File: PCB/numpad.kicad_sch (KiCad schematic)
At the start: 72 parts, among them J1 AVR-ISP-6, J2 Conn_01x04_Female, SW1 SW_Push, U1 ProMicro

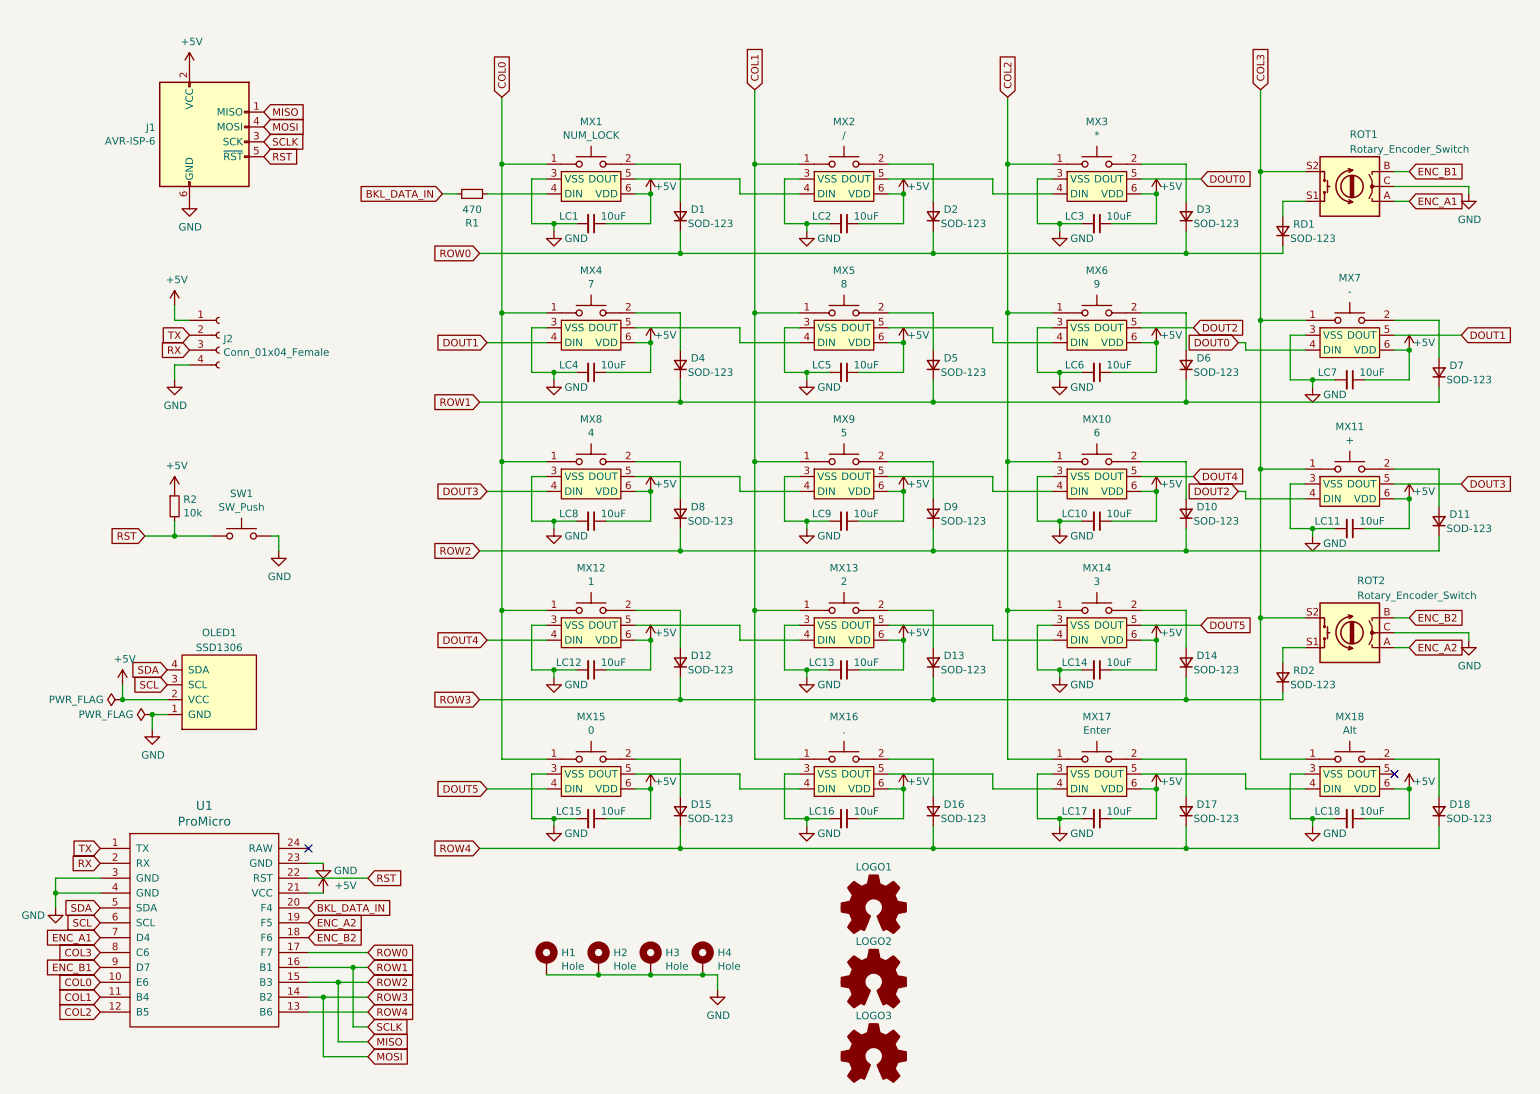
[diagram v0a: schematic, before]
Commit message: Completely redid schematic and PCB
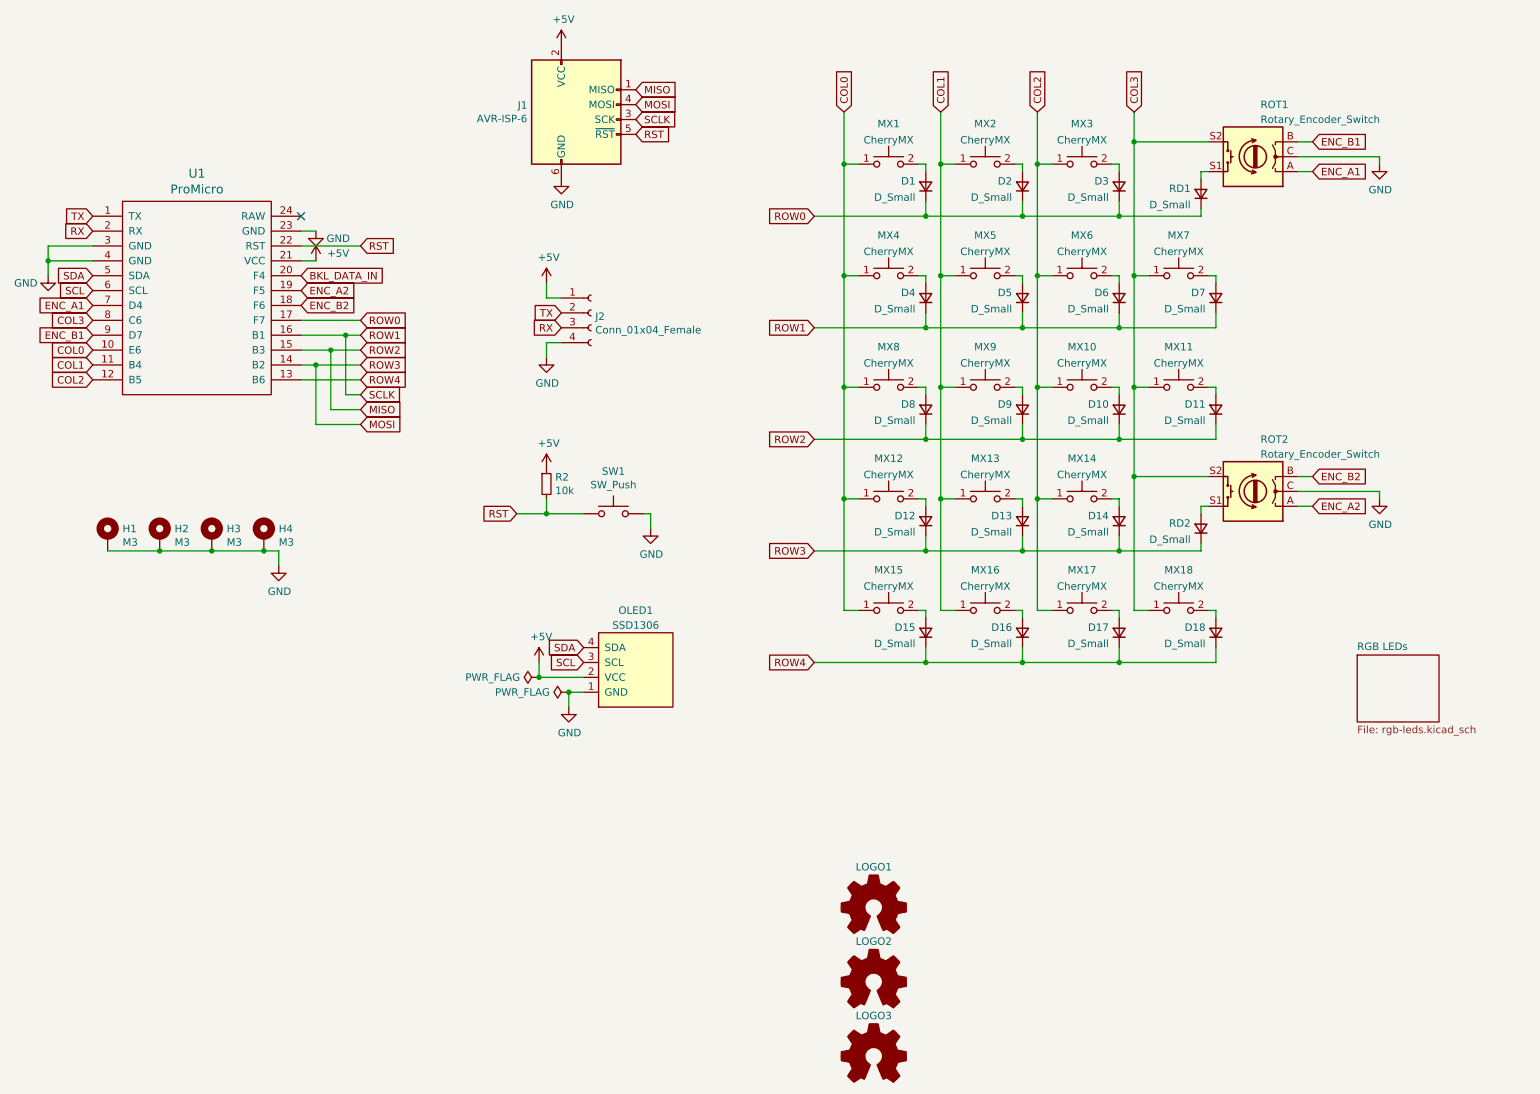
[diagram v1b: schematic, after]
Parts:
- removed LC1, LC10, LC11, LC12, LC13, LC14, LC15, LC16, LC17, LC18, LC2, LC3, LC4, LC5, LC6, LC7, LC8, LC9: 10uF, Capacitor_SMD:C_0805_2012Metric, symbol Device:C_Small
- removed MX1: NUM_LOCK, CherryMX_PCB_KailhSocket_LTST-A683CEGBW:CherryMX_1.00u_PCB_KailhSocket_LTST-A683CEGBW, symbol CherryMX:CherryMX_LTST-A683CEGBW
- removed MX10: 6, CherryMX_PCB_KailhSocket_LTST-A683CEGBW:CherryMX_1.00u_PCB_KailhSocket_LTST-A683CEGBW, symbol CherryMX:CherryMX_LTST-A683CEGBW
- removed MX11: +, CherryMX_PCB_KailhSocket_StabWireBottom_LTST-A683CEGBW:CherryMX_2.00u_PCB_KailhSocket_StabWireBottom_LTST-A683CEGBW, symbol CherryMX:CherryMX_LTST-A683CEGBW
- removed MX12: 1, CherryMX_PCB_KailhSocket_LTST-A683CEGBW:CherryMX_1.00u_PCB_KailhSocket_LTST-A683CEGBW, symbol CherryMX:CherryMX_LTST-A683CEGBW
- removed MX13: 2, CherryMX_PCB_KailhSocket_LTST-A683CEGBW:CherryMX_1.00u_PCB_KailhSocket_LTST-A683CEGBW, symbol CherryMX:CherryMX_LTST-A683CEGBW
- removed MX14: 3, CherryMX_PCB_KailhSocket_LTST-A683CEGBW:CherryMX_1.00u_PCB_KailhSocket_LTST-A683CEGBW, symbol CherryMX:CherryMX_LTST-A683CEGBW
- removed MX15: 0, CherryMX_PCB_KailhSocket_StabWireBottom_LTST-A683CEGBW:CherryMX_2.00u_PCB_KailhSocket_StabWireBottom_LTST-A683CEGBW, symbol CherryMX:CherryMX_LTST-A683CEGBW
- removed MX16: ., CherryMX_PCB_KailhSocket_LTST-A683CEGBW:CherryMX_1.00u_PCB_KailhSocket_LTST-A683CEGBW, symbol CherryMX:CherryMX_LTST-A683CEGBW
- removed MX17: Enter, CherryMX_PCB_KailhSocket_StabWireBottom_LTST-A683CEGBW:CherryMX_2.00u_PCB_KailhSocket_StabWireBottom_LTST-A683CEGBW, symbol CherryMX:CherryMX_LTST-A683CEGBW
- removed MX18: Alt, CherryMX_PCB_KailhSocket_LTST-A683CEGBW:CherryMX_1.50u_PCB_KailhSocket_LTST-A683CEGBW, symbol CherryMX:CherryMX_LTST-A683CEGBW
- removed MX2: /, CherryMX_PCB_KailhSocket_LTST-A683CEGBW:CherryMX_1.00u_PCB_KailhSocket_LTST-A683CEGBW, symbol CherryMX:CherryMX_LTST-A683CEGBW
- removed MX3: *, CherryMX_PCB_KailhSocket_LTST-A683CEGBW:CherryMX_1.00u_PCB_KailhSocket_LTST-A683CEGBW, symbol CherryMX:CherryMX_LTST-A683CEGBW
- removed MX4: 7, CherryMX_PCB_KailhSocket_LTST-A683CEGBW:CherryMX_1.00u_PCB_KailhSocket_LTST-A683CEGBW, symbol CherryMX:CherryMX_LTST-A683CEGBW
- removed MX5: 8, CherryMX_PCB_KailhSocket_LTST-A683CEGBW:CherryMX_1.00u_PCB_KailhSocket_LTST-A683CEGBW, symbol CherryMX:CherryMX_LTST-A683CEGBW
- removed MX6: 9, CherryMX_PCB_KailhSocket_LTST-A683CEGBW:CherryMX_1.00u_PCB_KailhSocket_LTST-A683CEGBW, symbol CherryMX:CherryMX_LTST-A683CEGBW
- removed MX7: -, CherryMX_PCB_KailhSocket_LTST-A683CEGBW:CherryMX_1.00u_PCB_KailhSocket_LTST-A683CEGBW, symbol CherryMX:CherryMX_LTST-A683CEGBW
- removed MX8: 4, CherryMX_PCB_KailhSocket_LTST-A683CEGBW:CherryMX_1.00u_PCB_KailhSocket_LTST-A683CEGBW, symbol CherryMX:CherryMX_LTST-A683CEGBW
- removed MX9: 5, CherryMX_PCB_KailhSocket_LTST-A683CEGBW:CherryMX_1.00u_PCB_KailhSocket_LTST-A683CEGBW, symbol CherryMX:CherryMX_LTST-A683CEGBW
- removed R1: 470, Resistor_SMD:R_0805_2012Metric, symbol Device:R_Small
- added MX1, MX10, MX12, MX13, MX14, MX16, MX2, MX3, MX4, MX5, MX6, MX7, MX8, MX9: CherryMX, CherryMX_PCB_KailhSocket:CherryMX_1.00u_PCB_KailhSocket, symbol CherryMX:CherryMX
- added MX11, MX17: CherryMX, CherryMX_PCB_KailhSocket_StabWireBottom:CherryMX_2.00u_PCB_KailhSocket_StabWireBottom, symbol CherryMX:CherryMX
- added MX15: CherryMX, CherryMX_PCB_KailhSocket_StabWireTop:CherryMX_2.00u_PCB_KailhSocket_StabWireTop, symbol CherryMX:CherryMX
- added MX18: CherryMX, CherryMX_PCB_KailhSocket:CherryMX_1.50u_PCB_KailhSocket, symbol CherryMX:CherryMX
- D1, D10, D11, D12, D13, D14, D15, D16, D17, D18, D2, D3, D4, D5, D6, D7, D8, D9: value SOD-123 -> D_Small; LCSC Part C2128 -> (none)
- H1, H2, H3, H4: value Hole -> M3
- R2: footprint Resistor_SMD:R_0805_2012Metric -> Resistor_SMD:R_0603_1608Metric
- RD1, RD2: value SOD-123 -> D_Small; footprint Diode_SMD:D_SOD-323_HandSoldering -> Diode_SMD:D_SOD-123; LCSC Part C2128 -> (none)
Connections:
- net COL0: now also MX1.1, MX12.1, MX15.1, MX4.1, MX8.1
- net COL1: now also MX13.1, MX16.1, MX2.1, MX5.1, MX9.1
- net COL2: now also MX10.1, MX14.1, MX17.1, MX3.1, MX6.1
- net COL3: now also MX11.1, MX18.1, MX7.1
- net at D4.2 (A): now also MX4.2
- net at D5.2 (A): now also MX5.2
- net at D6.2 (A): now also MX6.2
- net at D1.2 (A): now also MX1.2
- net at D2.2 (A): now also MX2.2
- net at D3.2 (A): now also MX3.2
- net at D8.2 (A): now also MX8.2
- net at D9.2 (A): now also MX9.2
- net at D10.2 (A): now also MX10.2
- net at D11.2 (A): now also MX11.2
- net at D7.2 (A): now also MX7.2
- net at D12.2 (A): now also MX12.2
- net at D13.2 (A): now also MX13.2
- net at D14.2 (A): now also MX14.2
- net at D15.2 (A): now also MX15.2
- net at D16.2 (A): now also MX16.2
- net at D17.2 (A): now also MX17.2
- net at D18.2 (A): now also MX18.2
- no-connect marks 2 -> 1
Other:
- added sheet RGB LEDs (rgb-leds.kicad_sch)
- moved on the sheet: H1, H2, H3, H4, J1, J2, OLED1, R2, ROT2, SW1, U1
